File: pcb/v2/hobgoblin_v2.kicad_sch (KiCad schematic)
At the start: 46 parts, among them J1 5V, J2 RC2014EXT1, J3 RC2014EXT2, J5 USBUART, SW1 RESET, SW2 ROMBNK, U1 74LS32, U10 MC68B50, U2 74LS14, U3 Z80CPU, U4 GAL16V8/IO, U6 628128, U7 74HCT00, U8 SST39SF010, U9 GAL16V8/MEM, X1 10MHz, X2 7.3728MHz

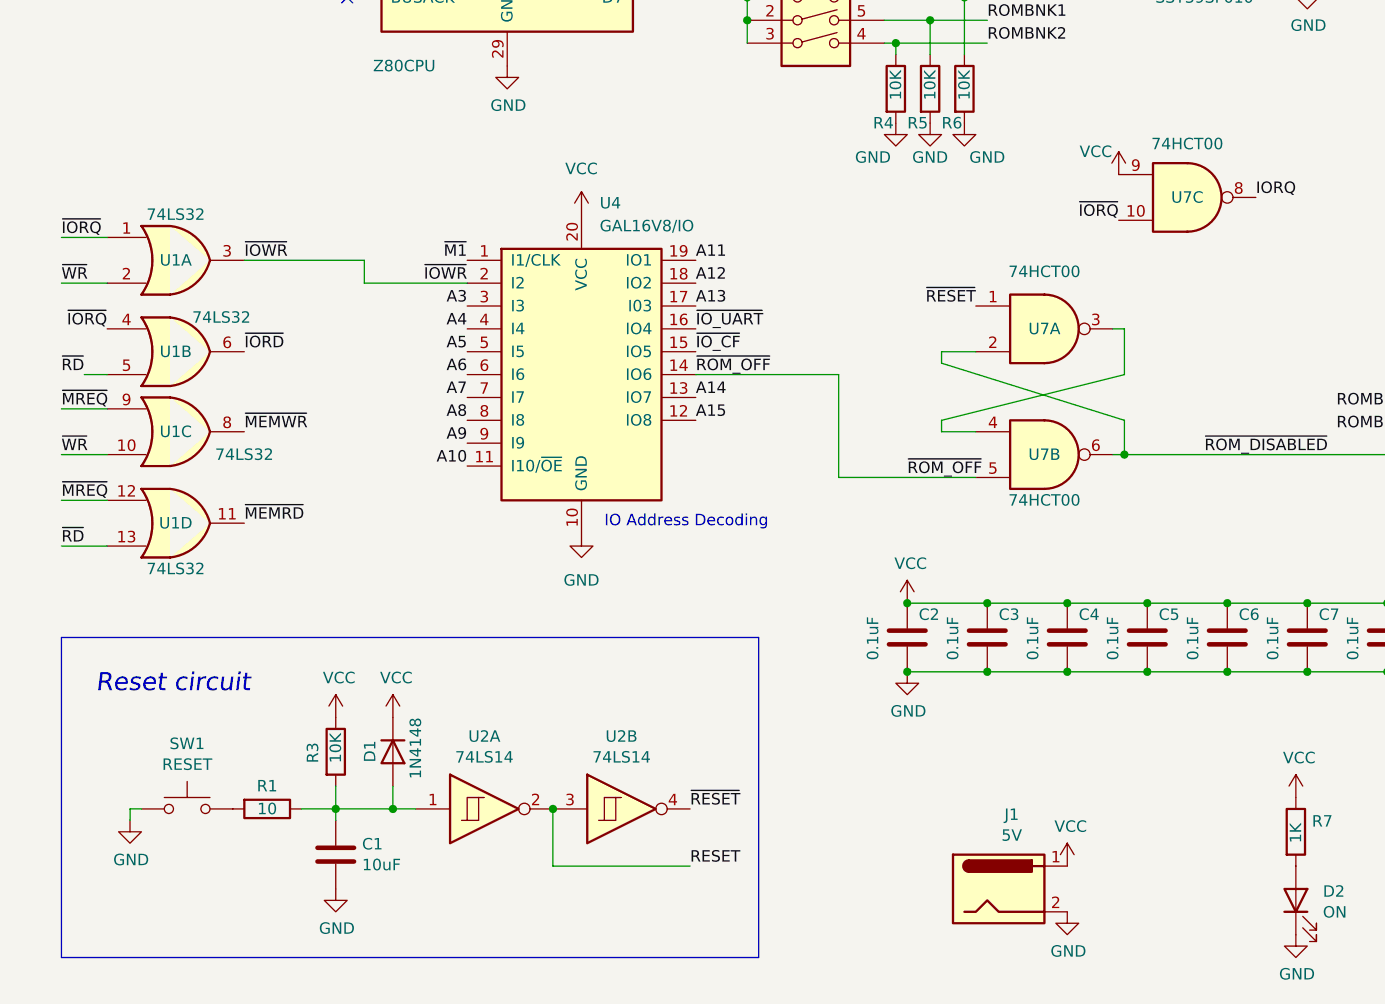
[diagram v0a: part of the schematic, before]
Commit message: Update to latest KiCAD version
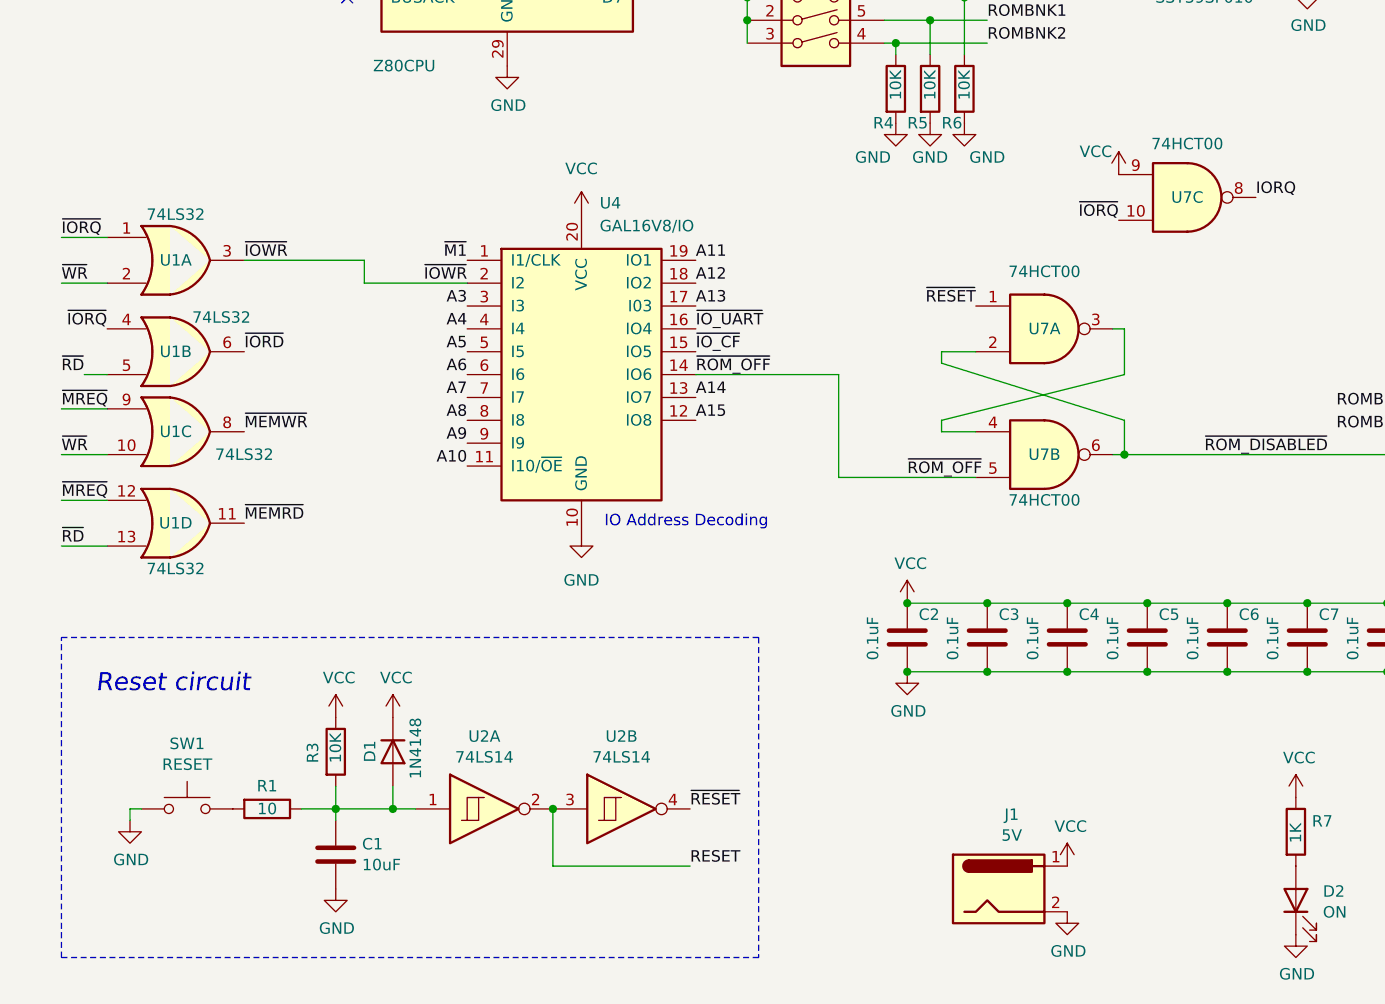
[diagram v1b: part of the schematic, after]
